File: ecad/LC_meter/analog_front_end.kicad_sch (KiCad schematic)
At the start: 36 parts, among them Q1 2N7000, Q2 2N7000, U1 LMC6484, U2 LMC6482, U3 LM385BZ-2.5, U4 MCP3204, U7 LMC6484

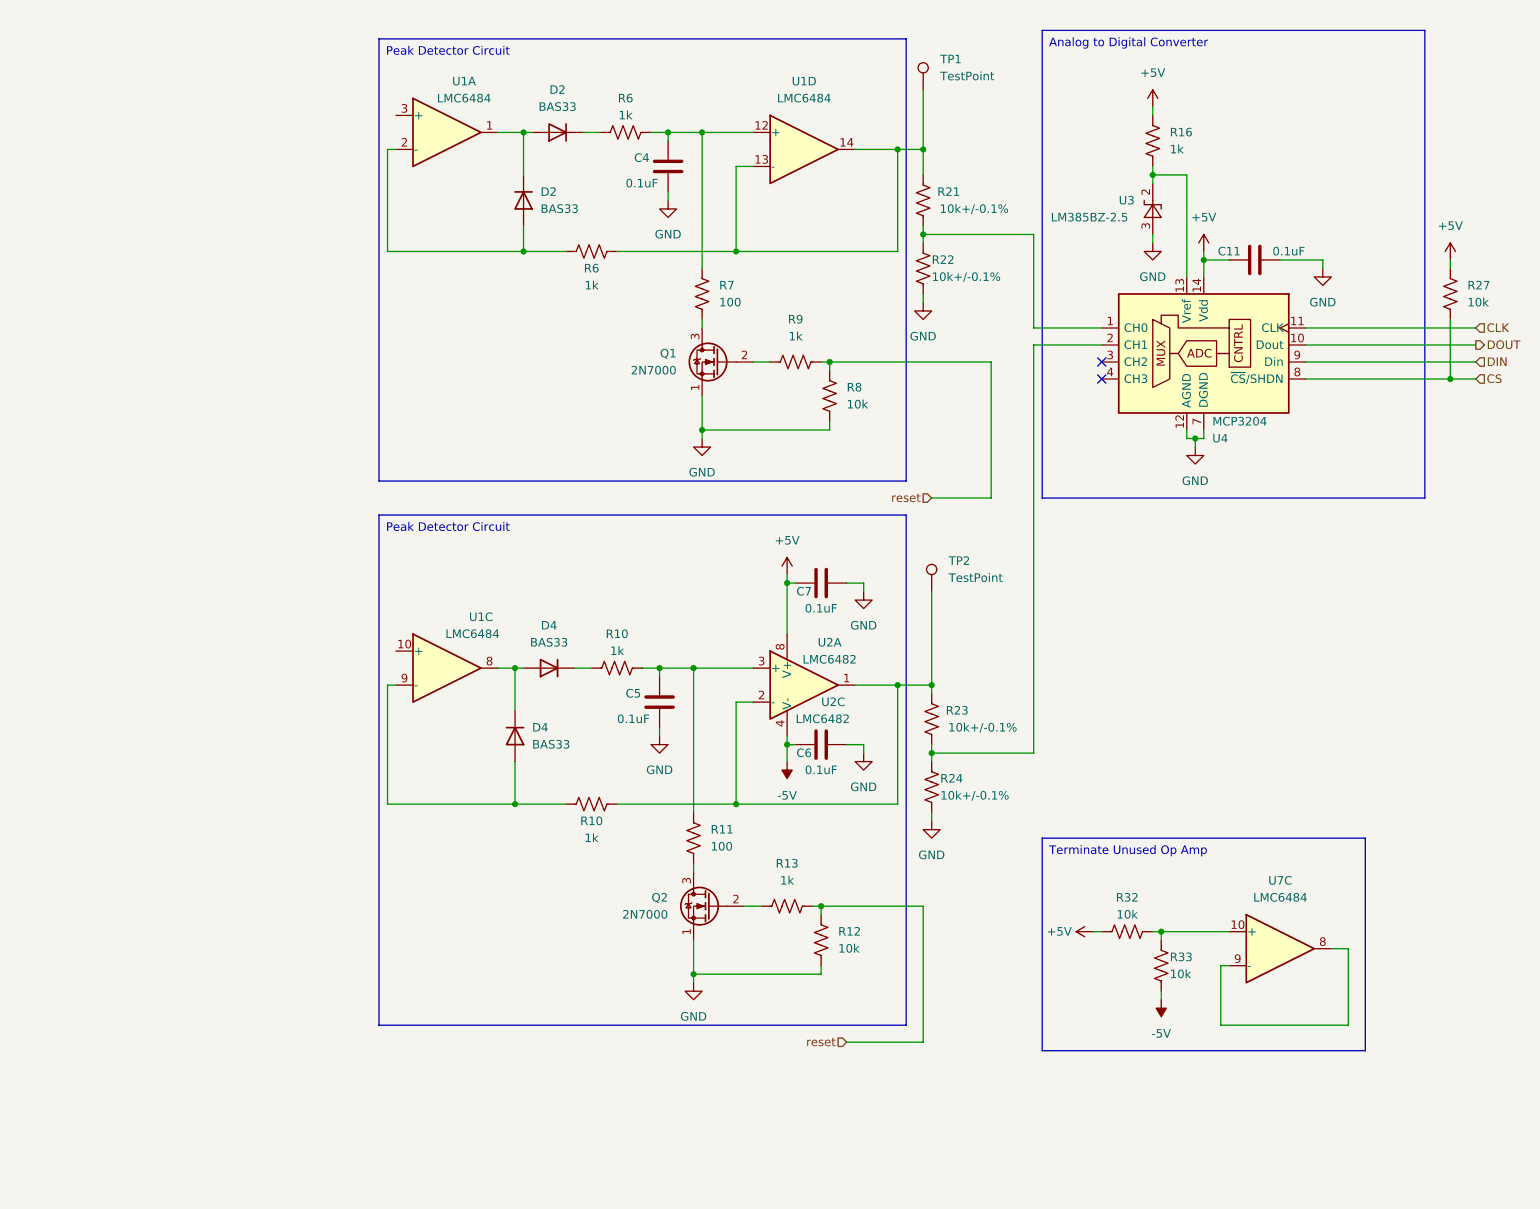
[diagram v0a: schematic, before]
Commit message: ok range calcs and schematic
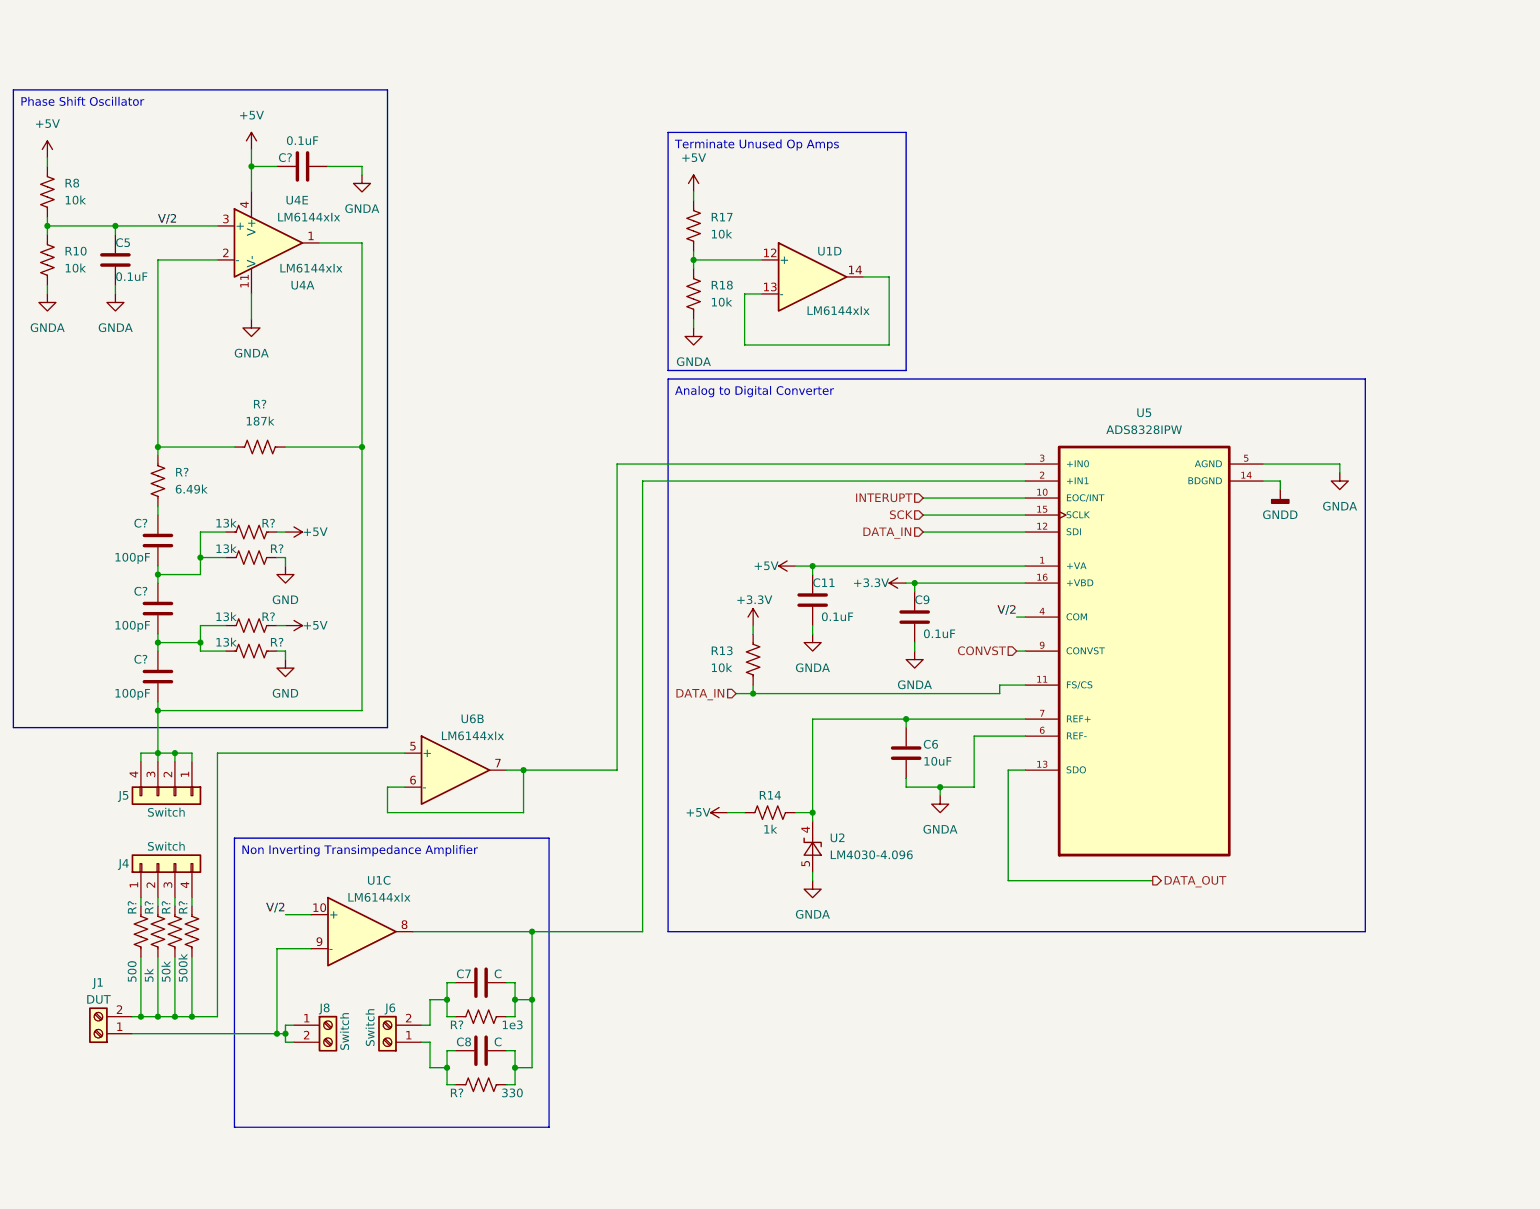
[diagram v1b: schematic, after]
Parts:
- removed C4: 0.1uF, symbol Device:C
- removed D2 (x2), D4 (x2): BAS33, symbol Device:D
- removed Q1, Q2: 2N7000, Package_TO_SOT_THT:TO-92_Inline, symbol Transistor_FET:2N7000
- removed R10 (x2), R16, R6 (x2), R9: 1k, symbol Device:R_US
- removed R11, R7: 100, symbol Device:R_US
- removed R12, R27, R32, R33: 10k, symbol Device:R_US
- removed R21, R22, R23, R24: 10k+/-0.1%, symbol Device:R_US
- removed TP1, TP2: TestPoint, symbol Connector:TestPoint
- removed U1, U7: LMC6484, symbol Amplifier_Operational:LMC6484
- removed U2: LMC6482, symbol Amplifier_Operational:LMC6482
- removed U3: LM385BZ-2.5, Package_TO_SOT_THT:TO-92_Inline, symbol Reference_Voltage:LM385BZ-2.5
- removed U4: MCP3204, symbol Analog_ADC:MCP3204
- added C8: C, symbol Device:C
- added C9, C?: 0.1uF, symbol Device:C
- added C? (x3): 100pF, symbol Device:C
- added J1: DUT, symbol Connector:Screw_Terminal_01x02
- added J4, J5: Switch, symbol Connector_Generic:Conn_01x04
- added J6, J8: Switch, symbol Connector:Screw_Terminal_01x02
- added R10, R17, R18: 10k, symbol Device:R_US
- added R14: 1k, symbol Device:R_US
- added R?: 187k, symbol Device:R_US
- added R? (x4): 13k, symbol Device:R_US
- added R?: 50k, symbol Device:R_US
- added R?: 330, symbol Device:R_US
- added R?: 500k, symbol Device:R_US
- added R?: 5k, symbol Device:R_US
- added R?: 500, symbol Device:R_US
- added R?: 1e3, symbol Device:R_US
- added R?: 6.49k, symbol Device:R_US
- added U1, U4, U6: LM6144xIx, symbol Amplifier_Operational:LM6144xIx
- added U2: LM4030-4.096, Package_TO_SOT_SMD:SOT-23-5, symbol Reference_Voltage:LM4030-4.096
- added U5: ADS8328IPW, ADS8328IPW:SOP65P640X120-16N, symbol LCR_parts:ADS8328IPW
- C6: value 0.1uF -> 10uF
- C7: value 0.1uF -> C
- R13: value 1k -> 10k
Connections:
- net +5V: now also R8.1, C?.1, R14.1, R17.1, R?.2, R?.2, U4.4 (V+), U5.1 (+VA); no longer C7.1
- net GND: now also R?.2, R?.2; no longer C11.2, C5.2, C6.2, C7.2, R8.2
- net V/2: now reaches C5.1
- net V/2: now also R8.2, R10.1, U1.10 (+), U4.3 (+), U5.4 (COM)
- net +3.3V: now reaches R13.1
- net +3.3V: now also C9.1, U5.16 (+VBD)
- net -5V: no longer names the net of C6.1
- net -5V: now also R14.2, U2.4 (K), U5.7 (REF+)
- net reset renamed DATA_IN
- net DATA_IN: now also U5.11 (FS/CS), U5.12 (SDI); no longer R8.1
- new net: C7.1, J6.2 (Pin_2), R?.1
- new net: C7.2, C8.2, R?.2, R?.2, U1.8, U5.2 (+IN1)
- new net: R?.1, R?.2, U4.2 (-)
- new net: C?.1, J5.1 (Pin_1), J5.2 (Pin_2), J5.3 (Pin_3), J5.4 (Pin_4), R?.2, U4.1
- new net: J1.1 (Pin_1), J8.1 (Pin_1), J8.2 (Pin_2), U1.9 (-)
- new net: J1.2 (Pin_2), R?.2, R?.2, R?.2, R?.2, U6.5 (+)
- new net: C?.1, C?.2, R?.1, R?.1 (x2)
- new net: R17.2, R18.1, U1.12 (+)
- new net: J4.3 (Pin_3), R?.1
- new net: C?.2, R?.1
- new net: U5.3 (+IN0), U6.6 (-), U6.7
- new net: C8.1, J6.1 (Pin_1), R?.1
- new net: J4.4 (Pin_4), R?.1
- new net: J4.2 (Pin_2), R?.1
- new net: J4.1 (Pin_1), R?.1
- new net: U1.13 (-), U1.14
- new net CONVST: U5.9 (CONVST)
- new net DATA_OUT: U5.13 (SDO)
- new net GNDA: C11.2, C5.2, C6.2, C9.2, C?.2, R10.2, R18.2, U2.5 (A), U4.11 (V-), U5.5 (AGND), U5.6 (REF-)
- new net GNDD: U5.14 (BDGND)
- new net INTERUPT: U5.10 (EOC/INT)
- new net SCK: U5.15 (SCLK)
- no-connect marks 2 -> 0

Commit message: crashed
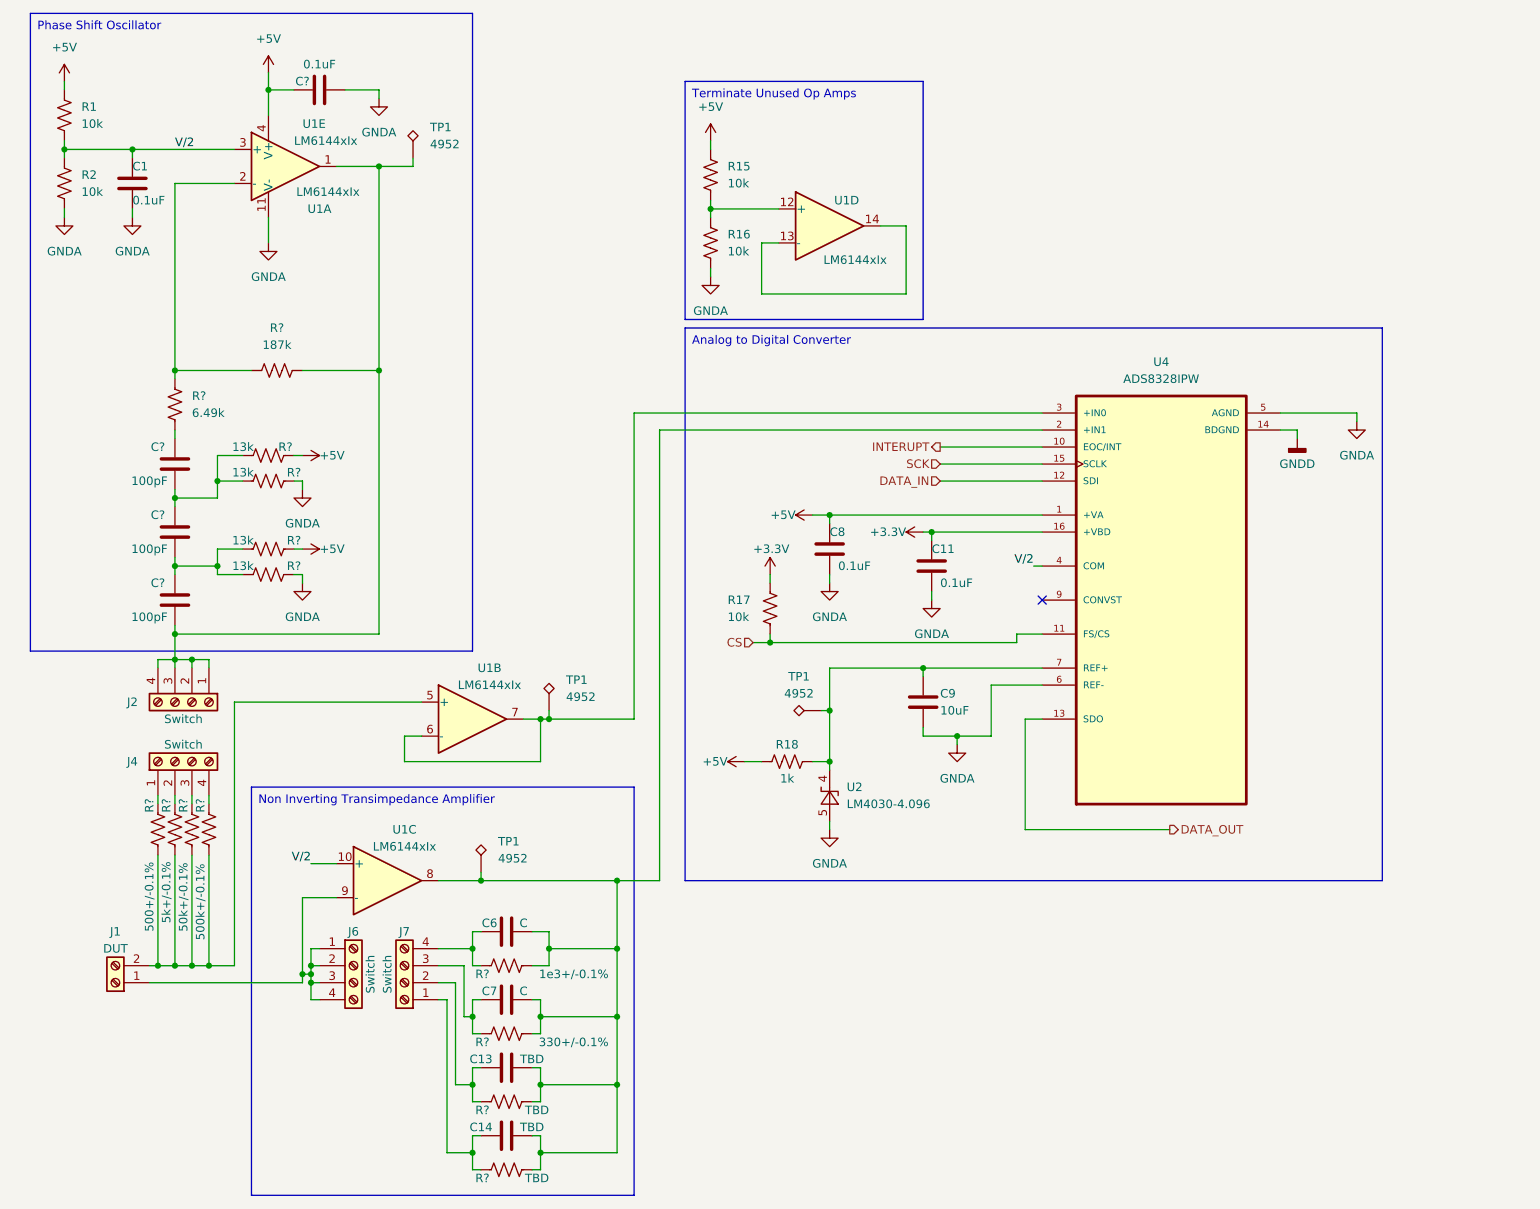
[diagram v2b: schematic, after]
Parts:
- removed J4, J5: Switch, symbol Connector_Generic:Conn_01x04
- removed J6, J8: Switch, symbol Connector:Screw_Terminal_01x02
- added C13, C14: TBD, Capacitor_SMD:C_0805_2012Metric, symbol Device:C
- added J2, J4, J6, J7: Switch, TerminalBlock_Phoenix:TerminalBlock_Phoenix_MPT-0,5-4-2.54_1x04_P2.54mm_Horizontal, symbol Connector:Screw_Terminal_01x04
- added R? (x2): TBD, Resistor_SMD:R_0805_2012Metric, symbol Device:R_US
- added TP1 (x4): 4952, Connector_Pin:Pin_D1.2mm_L10.2mm_W2.9mm_FlatFork, symbol Connector:TestPoint_Alt
- C1: renamed from C5; footprint (none) -> Capacitor_SMD:C_0805_2012Metric
- C11: renamed from C9; footprint (none) -> Capacitor_SMD:C_0805_2012Metric
- C6: renamed from C7; footprint (none) -> Capacitor_SMD:C_0805_2012Metric
- C7: renamed from C8; footprint (none) -> Capacitor_SMD:C_0805_2012Metric
- C8: renamed from C11; footprint (none) -> Capacitor_SMD:C_0805_2012Metric
- C9: renamed from C6; footprint (none) -> Capacitor_SMD:C_0805_2012Metric
- C? (x4): footprint (none) -> Capacitor_SMD:C_0805_2012Metric
- J1: footprint (none) -> TerminalBlock_Phoenix:TerminalBlock_Phoenix_MPT-0,5-2-2.54_1x02_P2.54mm_Horizontal
- R1: renamed from R8; footprint (none) -> Resistor_SMD:R_0805_2012Metric
- R15: renamed from R17; footprint (none) -> Resistor_SMD:R_0805_2012Metric
- R16: renamed from R18; footprint (none) -> Resistor_SMD:R_0805_2012Metric
- R17: renamed from R13; footprint (none) -> Resistor_SMD:R_0805_2012Metric
- R18: renamed from R14; footprint (none) -> Resistor_SMD:R_0805_2012Metric
- R2: renamed from R10; footprint (none) -> Resistor_SMD:R_0805_2012Metric
- R? (x6): footprint (none) -> Resistor_SMD:R_0805_2012Metric
- R?: value 50k -> 50k+/-0.1%; footprint (none) -> Resistor_SMD:R_0805_2012Metric
- R?: value 330 -> 330+/-0.1%; footprint (none) -> Resistor_SMD:R_0805_2012Metric
- R?: value 500k -> 500k+/-0.1%; footprint (none) -> Resistor_SMD:R_0805_2012Metric
- R?: value 5k -> 5k+/-0.1%; footprint (none) -> Resistor_SMD:R_0805_2012Metric
- R?: value 500 -> 500+/-0.1%; footprint (none) -> Resistor_SMD:R_0805_2012Metric
- R?: value 1e3 -> 1e3+/-0.1%; footprint (none) -> Resistor_SMD:R_0805_2012Metric
- U1: renamed from U4; footprint (none) -> Package_DIP:DIP-14_W7.62mm
- U1: footprint (none) -> Package_DIP:DIP-14_W7.62mm
- U1: renamed from U6; footprint (none) -> Package_DIP:DIP-14_W7.62mm
- U4: renamed from U5; footprint ADS8328IPW:SOP65P640X120-16N -> Package_SO:TSSOP-14-1EP_4.4x5mm_P0.65mm
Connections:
- net GND is gone; now on net GNDA: R?.2, R?.2
- net DATA_IN: no longer R17.2, U4.11 (FS/CS)
- net at C9.1, R18.2, U2.4 (K)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: now also TP1.1
- net at C6.1, R?.1: now also J7.4 (Pin_4)
- net at C6.2, C7.2, R?.2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: now also C13.2, C14.2, R?.2, R?.2, TP1.1
- net at C?.1, R?.2, U1.1: now also J2.1 (Pin_1), J2.2 (Pin_2), J2.3 (Pin_3), J2.4 (Pin_4), TP1.1
- net at J1.1 (Pin_1), U1.9 (-): now also J6.1 (Pin_1), J6.2 (Pin_2), J6.3 (Pin_3), J6.4 (Pin_4)
- net at R?.1: now also J4.3 (Pin_3)
- net at U1.6 (-), U1.7, U4.3 (+IN0): now also TP1.1
- net at C7.1, R?.1: now also J7.3 (Pin_3)
- net at R?.1: now also J4.4 (Pin_4)
- net at R?.1: now also J4.2 (Pin_2)
- net at R?.1: now also J4.1 (Pin_1)
- net CONVST: no longer names the net of U4.9 (CONVST)
- new net: C14.1, J7.1 (Pin_1), R?.1
- new net: C13.1, J7.2 (Pin_2), R?.1
- new net CS: R17.2, U4.11 (FS/CS)
- no-connect marks 0 -> 1
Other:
- moved on the sheet: C1, C11, C6, C7, C8, C9, C?, J1, R1, R15, R16, R17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
